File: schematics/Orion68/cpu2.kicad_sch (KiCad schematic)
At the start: 37 parts, among them J10 Conn_02x08_Counter_Clockwise, J600 Euro96pin, J601 clock, J602 clock1, Q5 2N3904, Q6 2N3904, SW1 sw_reset, U16 74LS139, U21 74LS20, U22 74HC164, U24 74HC4078, U600 68000D, U601 74LS393, U602 74HC74, U603 74HC14, U604 ATmega8-16P

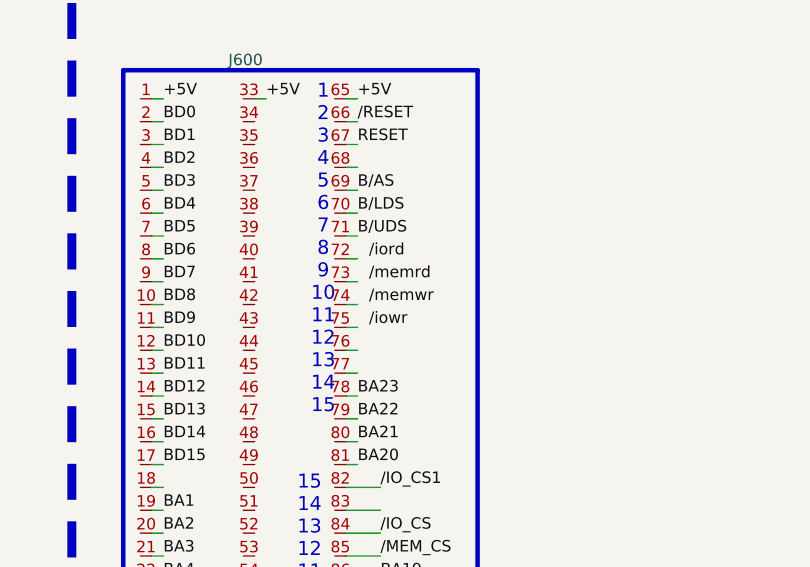
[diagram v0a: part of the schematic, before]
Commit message: just update
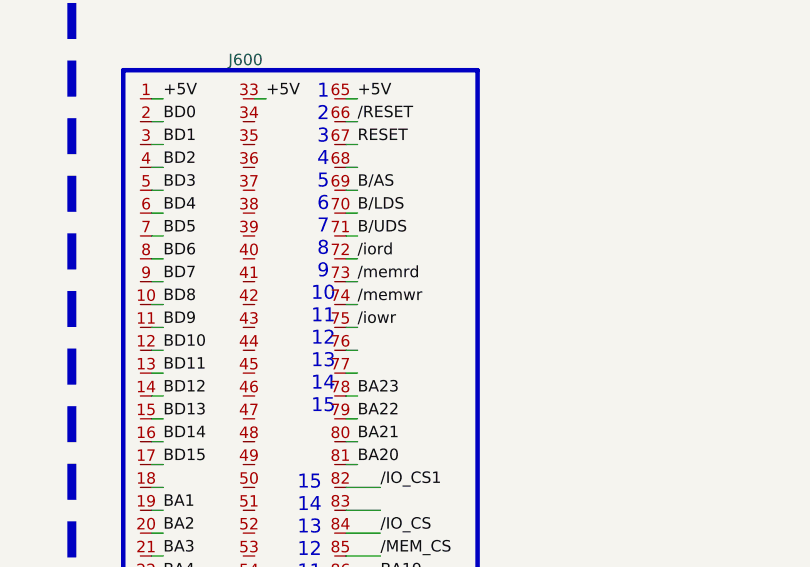
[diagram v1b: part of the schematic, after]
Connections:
- net R/W: now also J600.74
- net /iord: now also J600.72
- net /iowr: now also J600.75
- net /memrd: now also J600.73
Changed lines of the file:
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@@
 	)
 	(label "{slash}memrd"
-		(at 265.43 63.5 0)
+		(at 264.16 63.5 0)
 		(effects
 			(font
@@
 	)
 	(label "{slash}memwr"
-		(at 265.43 66.04 0)
+		(at 264.16 66.04 0)
 		(effects
 			(font
@@
 	)
 	(label "{slash}iowr"
-		(at 265.43 68.58 0)
+		(at 264.16 68.58 0)
 		(effects
 			(font
@@
 	)
 	(label "{slash}iord"
-		(at 265.43 60.96 0)
-		(effects
-			(font
+		(at 264.16 60.96 0)
+		(effects
+			(font
